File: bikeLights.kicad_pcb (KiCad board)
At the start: 2 copper layers, 71.1 x 66 mm, 24 parts, among them J1 Battery, J2 Light Sensor, J3 Front Light, J4 Rear Lights, J5 Hub Power In, Q1 IRF9540N, Q2 P2N2222A, Q3 RFP30N06LE, Q4 P2N2222A

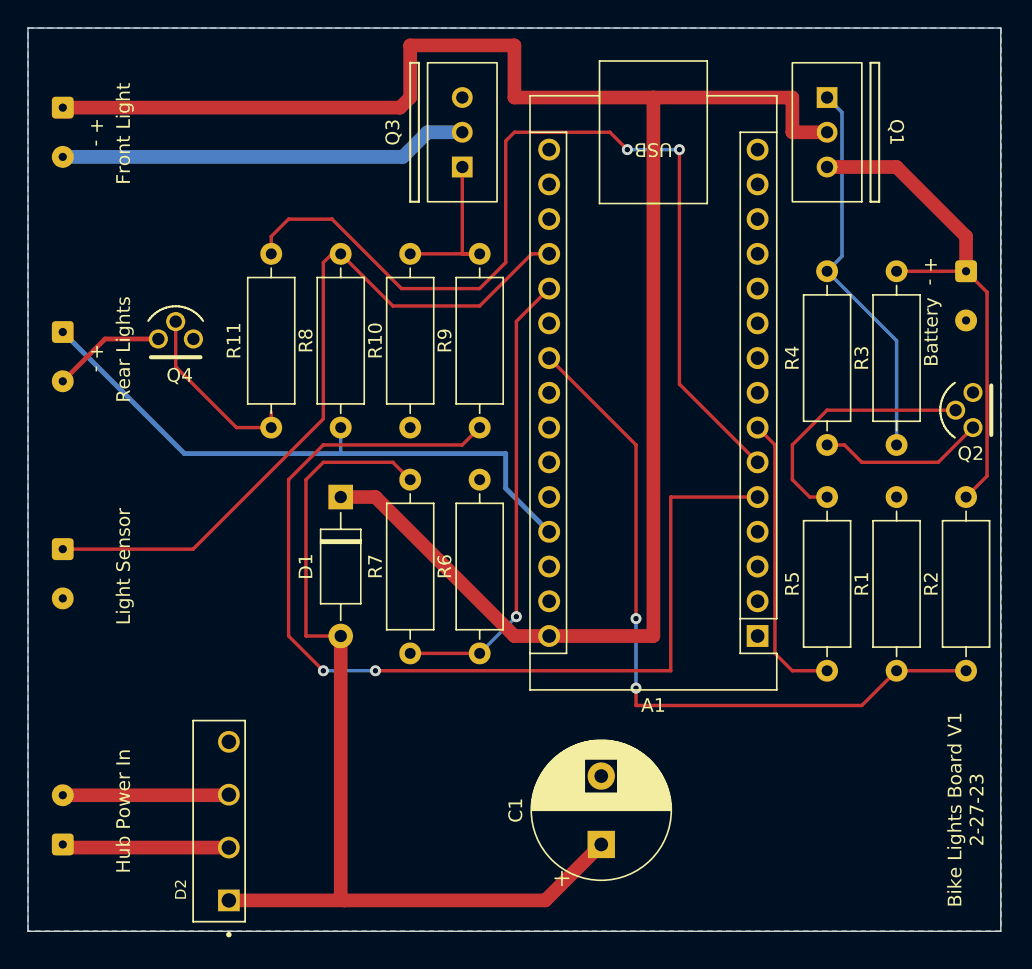
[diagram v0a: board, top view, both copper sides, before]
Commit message: updates
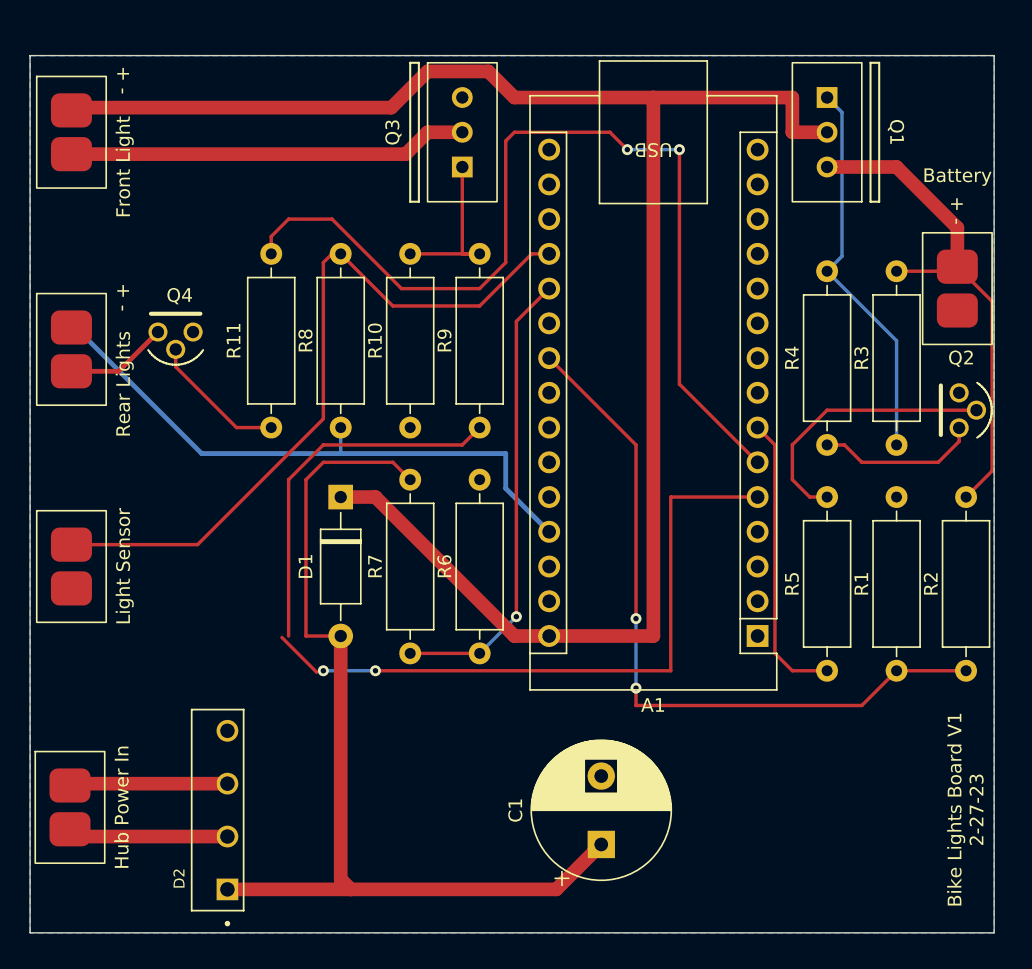
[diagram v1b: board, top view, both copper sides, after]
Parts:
- J1, J2, J3, J4, J5: footprint Connector_Wire:SolderWire-0.1sqmm_1x02_P3.6mm_D0.4mm_OD1mm -> solder_pads:solder_pads_medium
- moved J5 2.76 mm to (93.2, 126.8), turned to -90 degrees
- moved J3 1.91 mm to (93.3, 77.5)
- moved J1 1.42 mm to (158.1, 88.9)
- moved J2 1.42 mm to (93.3, 109.2)
- moved J4 1.42 mm to (93.3, 93.3)
- moved D2 0.81 mm to (104.7, 132.8)
- moved Q4 0.51 mm to (101.0, 92.6), turned to 90 degrees
- turned Q2 to 180 degrees
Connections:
- Q2 pad 1: Net-(Q2-Pad1) -> GND
- Q2 pad 3: GND -> Net-(Q2-Pad3)
- Q4 pad 1: Net-(J4-Pad2) -> GND
- Q4 pad 3: GND -> Net-(J4-Pad2)
- R4 pad 2: Net-(Q2-Pad1) -> Net-(Q2-Pad3)
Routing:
- net Net-(Q2-Pad1): track 12.2 -> 0.00 mm
- net Net-(Q2-Pad3): track 0.00 -> 11.8 mm
- net Net-(A1-Pad30): track 132.8 -> 126.2 mm
- net Net-(Q4-Pad2): track 13.3 -> 10.1 mm
- net Net-(Q2-Pad2): track 18.6 -> 20.1 mm
- net GND: track 1.22 -> 0.00 mm
- net Net-(C1-Pad1): track 71.0 -> 70.2 mm
- net Net-(A1-Pad19): track 54.4 -> 53.6 mm
- net Net-(J4-Pad2): track 8.27 -> 7.51 mm
- net Net-(J3-Pad2): track 30.0 -> 29.2 mm
- net Net-(D2-Pad3): track 12.2 -> 11.6 mm
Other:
- board size 71.1 x 66 mm -> 70.5 x 64.1 mm
